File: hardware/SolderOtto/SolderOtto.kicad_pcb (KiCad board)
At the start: 4 copper layers, 121 x 60 mm, 224 parts, among them J201 Conn_02x04_Counter_Clockwise, J301 TC-2050, J401 Conn_01x20, J501 Conn_01x08, J601 Conn_01x07, P301 USB_C_Plug_USB2.0, Q201 T2N7002AK, Q202 BC858B, Q203 BC847A, Q204 BC847A, Q801 Q_Dual_NMOS, Q802 Q_Dual_NMOS, Q803 Q_Dual_NMOS, Q804 DTD123EK, Q805 DTD123EK, Q806 DTD123EK, Q807 Q_Dual_NMOS, Q808 Q_Dual_NMOS, Q809 DTD123EK, Q810 DTD123EK, Q901 BC847A, Q902 BC858B, Q903 BC847A, SW301 SW_Push, U201 LM5012, U202 AP3211K, U203 AP3211K, U204 AP3211K, U205 LM27761, U206 MCP9701T-E/TT, U301 USBLC6-2SC6, U302 STM32G474QETx, U303 MX25R3235FM1xx0, U701 SN74LVC125A, U702 TS5A3159ADCK, U801 VOM1271, U802 VOM1271, U803 VOM1271, U804 VOM1271, U805 VOM1271, U901 OPA202, U902 LM358B, U903 74hc4053, U904 OPA202, U905 OPA202, Y301 32.768 kHz

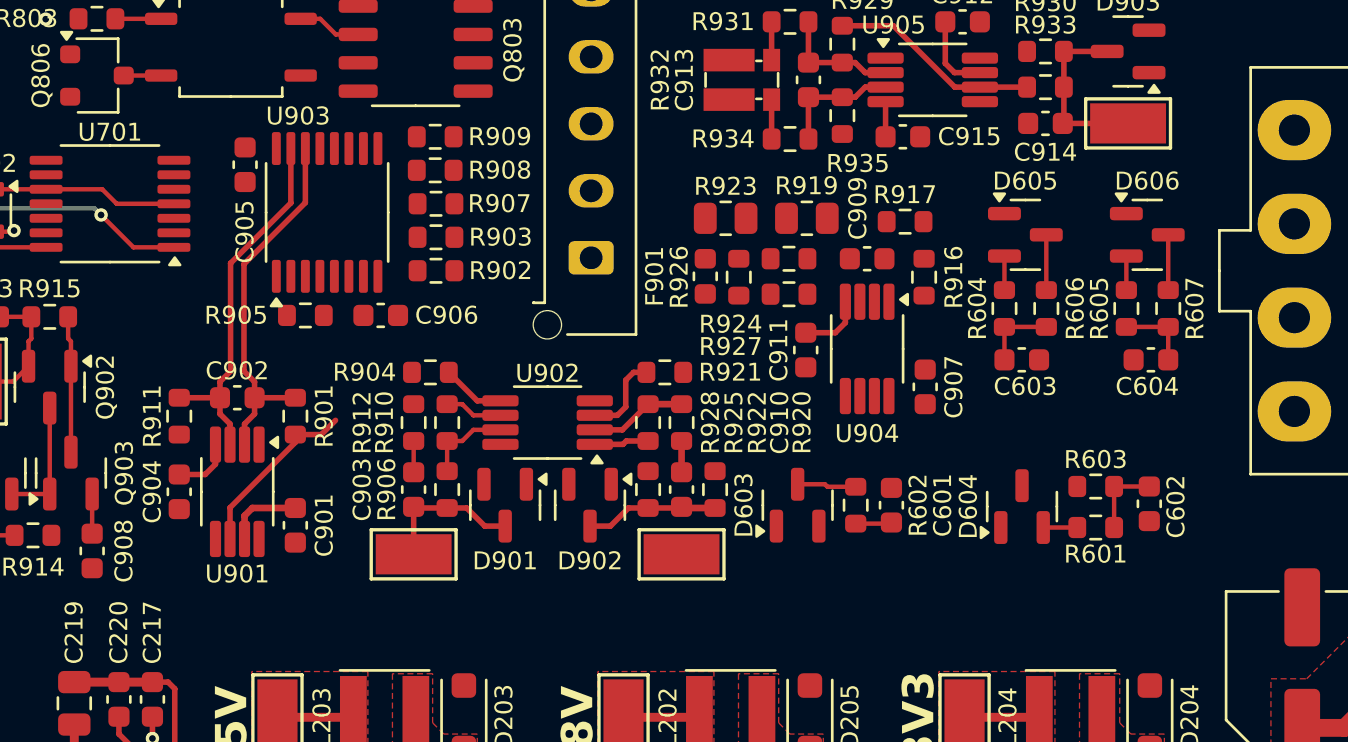
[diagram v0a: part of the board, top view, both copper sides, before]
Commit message: save work
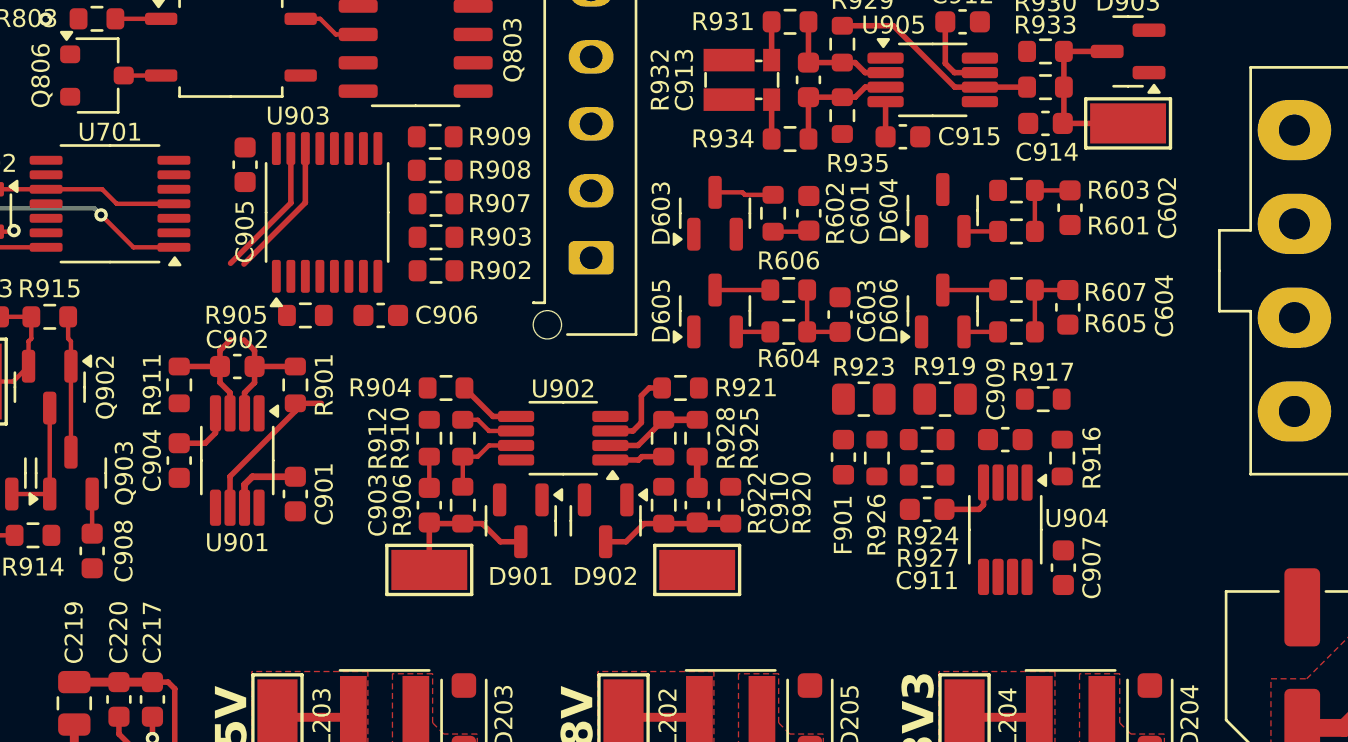
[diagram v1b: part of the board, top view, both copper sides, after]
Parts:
- moved D605 14.3 mm to (144.8, 79.8), turned to 90 degrees
- moved C602 13.7 mm to (160.7, 75.2)
- moved D604 13.7 mm to (155.0, 75.3)
- moved R601 13.7 mm to (158.3, 76.2)
- moved R603 13.7 mm to (158.3, 74.4)
- moved C601 13.6 mm to (149.0, 75.4)
- moved D603 13.6 mm to (144.8, 75.4)
- moved R602 13.6 mm to (147.4, 75.4)
- moved R606 11.6 mm to (148.1, 78.9), turned to 0 degrees
- moved R916 10.2 mm to (160.3, 86.4)
- moved R926 10.2 mm to (152.1, 86.4)
- moved R927 10.2 mm to (154.3, 87.2)
- moved C907 10.2 mm to (160.4, 91.3)
- moved C909 10.2 mm to (157.8, 85.6)
- moved F901 10.2 mm to (150.6, 86.3)
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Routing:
- net Net-(U901A-+): track 16.6 -> 11.8 mm
- net /Channel0/channel_meas/IN-: track 16.6 -> 11.8 mm
- net Net-(R901-Pad2): track 7.95 -> 7.05 mm
